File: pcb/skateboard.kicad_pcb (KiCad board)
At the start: 4 copper layers, 83.6 x 84.8 mm, 186 parts, among them J1 RC555, J10 PH_2.0, J11 adc_sensor2, J12 adc_sensor1, J13 Conn_01x01_Pin, J14 Conn_01x01_Pin, J15 Conn_01x01_Pin, J16 Conn_01x01_Pin, J17 Conn_01x02_Pin, J2 pa1010d, J3 can_sensor, J4 USB_C_Receptacle_USB2.0_16P, J5 UART, J6 TB_MOTOR, J7 PH_2.0, J8 power, J9 TB_MOTOR, Q1 AO3401A, Q4 BTN8982TA, Q5 BTN8982TA, Q6 BTN8982TA, Q7 BTN8982TA, Q8 BTN8982TA, Q9 BTN8982TA, SW1 SW_SPST, SW2 BOOT, SW3 EN, U1 HX711, U10 INA240A2PW, U11 INA240A2PW, U2 SIT1042AQT/3, U3 ESP32-S3-WROOM-1, U4 LMR16030SDDAR, U5 LMR16030SDDAR, U6 LMR16030SDDAR, U7 INA240A2PW, U8 INA240A2PW, U9 HX711

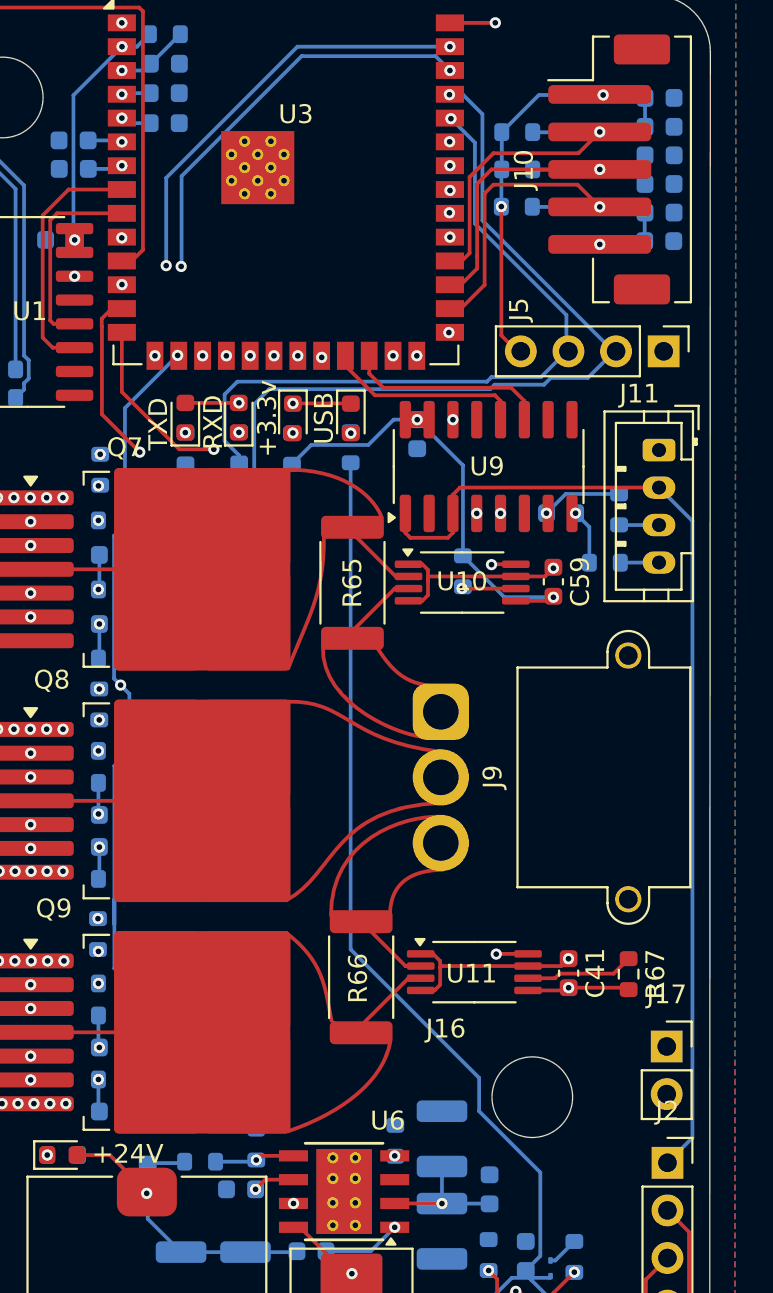
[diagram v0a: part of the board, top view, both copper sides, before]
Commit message: feat: update
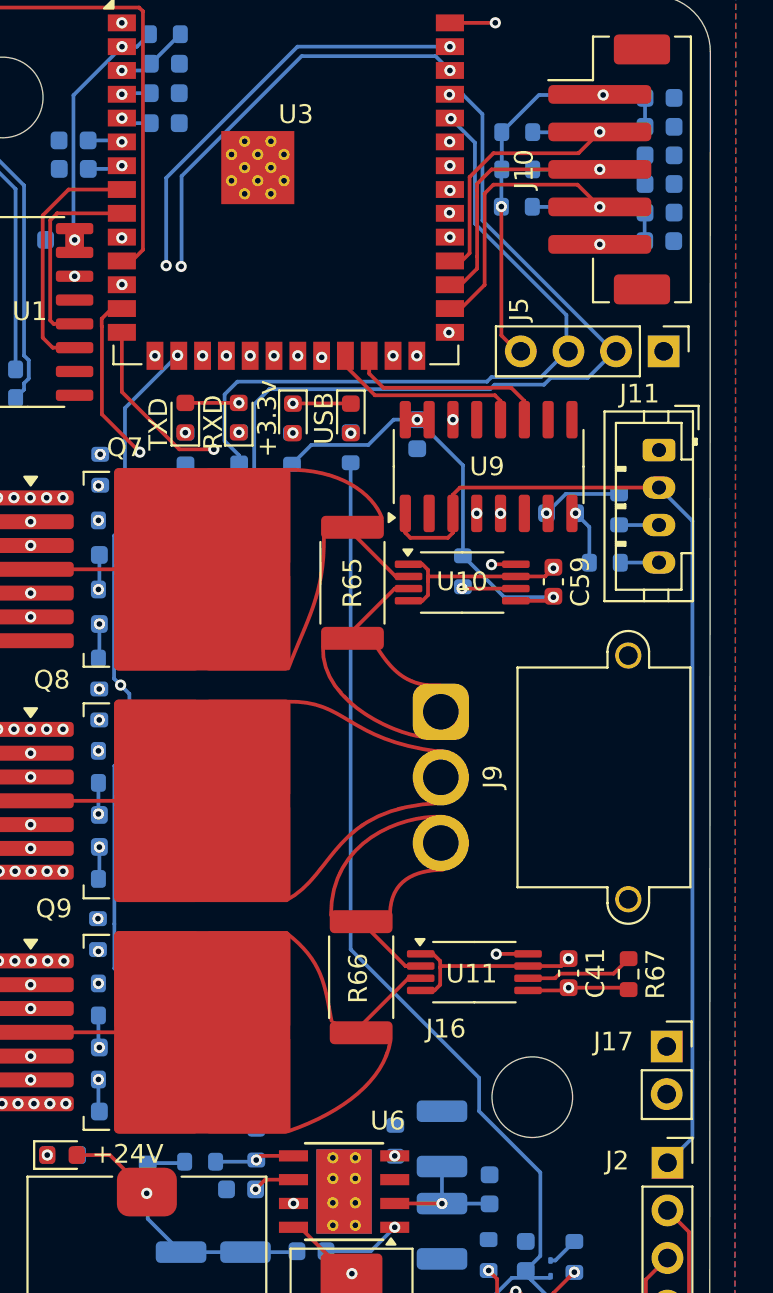
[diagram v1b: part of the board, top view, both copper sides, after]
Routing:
- net MOTO_POWER: track 85.8 -> 84.5 mm
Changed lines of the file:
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@@
 			(drillshape 0)
 			(scaleselection 1)
-			(outputdirectory "C:/Users/Aril Linda/Desktop/millionBoard/pcb/Gerber/")
+			(outputdirectory "C:/Users/Aril Linda/Desktop/millionBoard/pcb/Gerber")
 		)
 	)
@@
 		(tags "Through hole socket strip THT 1x02 2.54mm single row")
 		(property "Reference" "J17"
-			(at 0 -2.77 0)
+			(at -2.8448 -0.254 0)
 			(layer "F.SilkS")
 			(effects
@@
 		(tags "Through hole socket strip THT 1x05 2.54mm single row")
 		(property "Reference" "J2"
-			(at 0 -2.77 0)
+			(at -2.6812 -0.1088 0)
 			(layer "F.SilkS")
 			(effects
@@
 	)
 	(via
-		(at 140.505 83.52)
+		(at 140.5065 83.5215)
 		(size 0.6)
 		(drill 0.3)
@@
 	(segment
 		(start 140.775 83.79)
-		(end 140.505 83.52)
+		(end 140.5065 83.5215)
 		(width 0.2)
 		(layer "B.Cu")
@@
 	)
 	(segment
-		(start 122.3401 83.8654)
-		(end 121.7568 84.4487)
+		(start 140.5065 83.5215)
+		(end 140.505 83.52)
 		(width 0.2)
-		(layer "In2.Cu")
+		(layer "B.Cu")
 		(net 37)
 	)
 	(segment
-		(start 132.9133 85.322)
-		(end 131.4567 83.8654)
+		(start 138.555958 85.322)
+		(end 140.357957 83.52)
 		(width 0.2)
 		(layer "In2.Cu")
@@
 	)
 	(segment
-		(start 139.523379 84.354579)
-		(end 140.089957 83.788)
+		(start 122.3401 83.8654)
+		(end 121.7568 84.4487)
 		(width 0.2)
 		(layer "In2.Cu")
@@
 	)
 	(segment
-		(start 121.7568 91.449743)
-		(end 101.5492 111.657343)
+		(start 132.9133 85.322)
+		(end 131.4567 83.8654)
 		(width 0.2)
 		(layer "In2.Cu")
@@
 	)
 	(segment
-		(start 139.523379 84.354579)
-		(end 138.555958 85.322)
+		(start 121.7568 91.449743)
+		(end 101.5492 111.657343)
 		(width 0.2)
 		(layer "In2.Cu")
@@
 	)
 	(segment
-		(start 139.503 84.374957)
-		(end 139.523379 84.354579)
-		(width 0.2)
-		(layer "In2.Cu")
-		(net 37)
-	)
-	(segment
 		(start 101.5492 111.657343)
 		(end 101.5492 112.685729)
@@
 	)
 	(segment
-		(start 140.505 83.788)
+		(start 140.357957 83.52)
 		(end 140.505 83.52)
 		(width 0.2)
@@
 	)
 	(segment
-		(start 140.089957 83.788)
-		(end 140.505 83.788)
-		(width 0.2)
-		(layer "In2.Cu")
-		(net 37)
-	)
-	(segment
 		(start 161.5225 107.32)
 		(end 160.2436 107.32)
@@
 		(width 0.2)
 		(layer "B.Cu")
-		(net 134)
-	)
-	(segment
-		(start 140.104 125.19)
-		(end 140.104 126.51)
-		(width 0.2)
-		(layer "B.Cu")
